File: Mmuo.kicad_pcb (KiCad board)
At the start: 4 copper layers, 95 parts, among them IC1 A121-001-T&R, IC2 BQ24253RGER, IC3 ADPL40502AUJZ-1.8-R7, J1 USB_C_Receptacle_USB2.0_16P, J2 B2B-PH-K-S, J3 SW_Debug, Q1 BSS84, Q2 BSS138, Q3 MMBT3904, SW1 PTS815, U1 USBLC6-2SC6, U2 RT9166A-33GXL, U3 EKMB1309113K, U4 STM32WB55CGU6, U5 MCP9808_MSOP, Y1 24MHz, Y2 32MHz, Y3 32K768

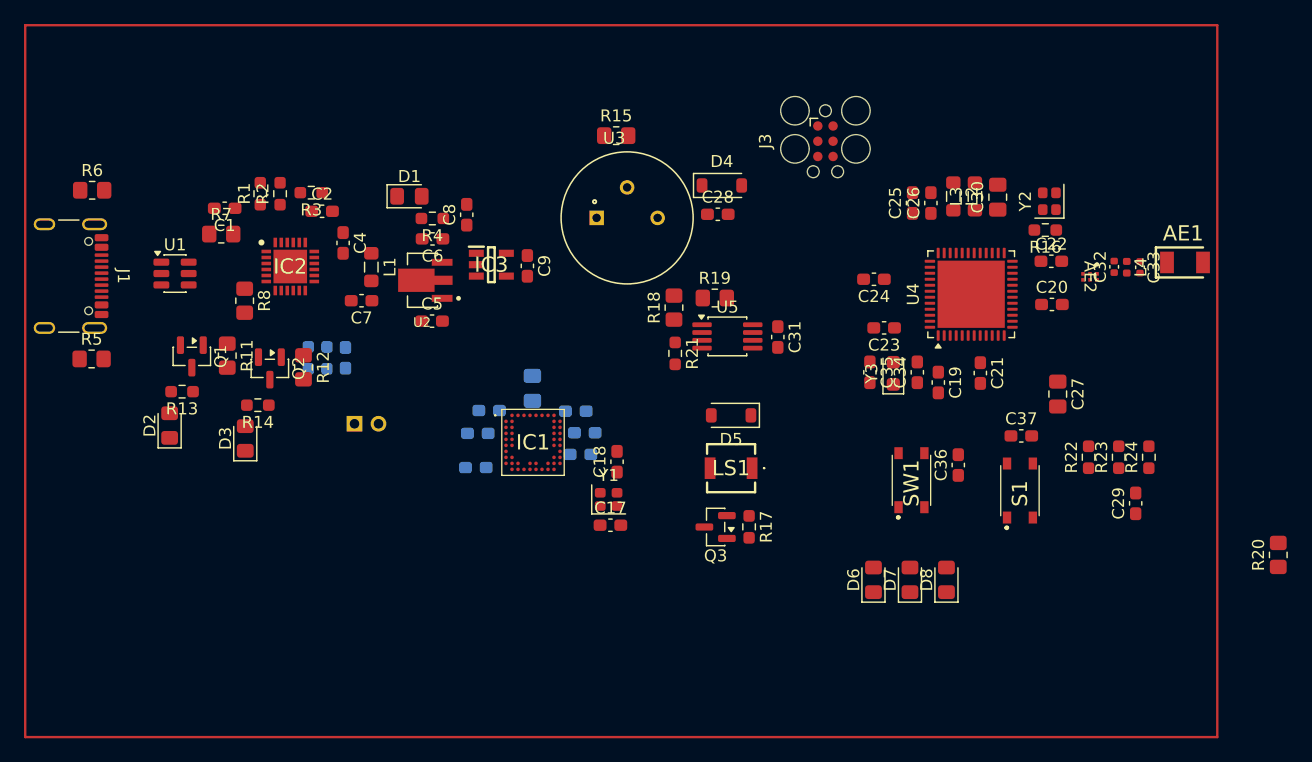
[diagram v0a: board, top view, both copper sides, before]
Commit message: Layout and initial routing
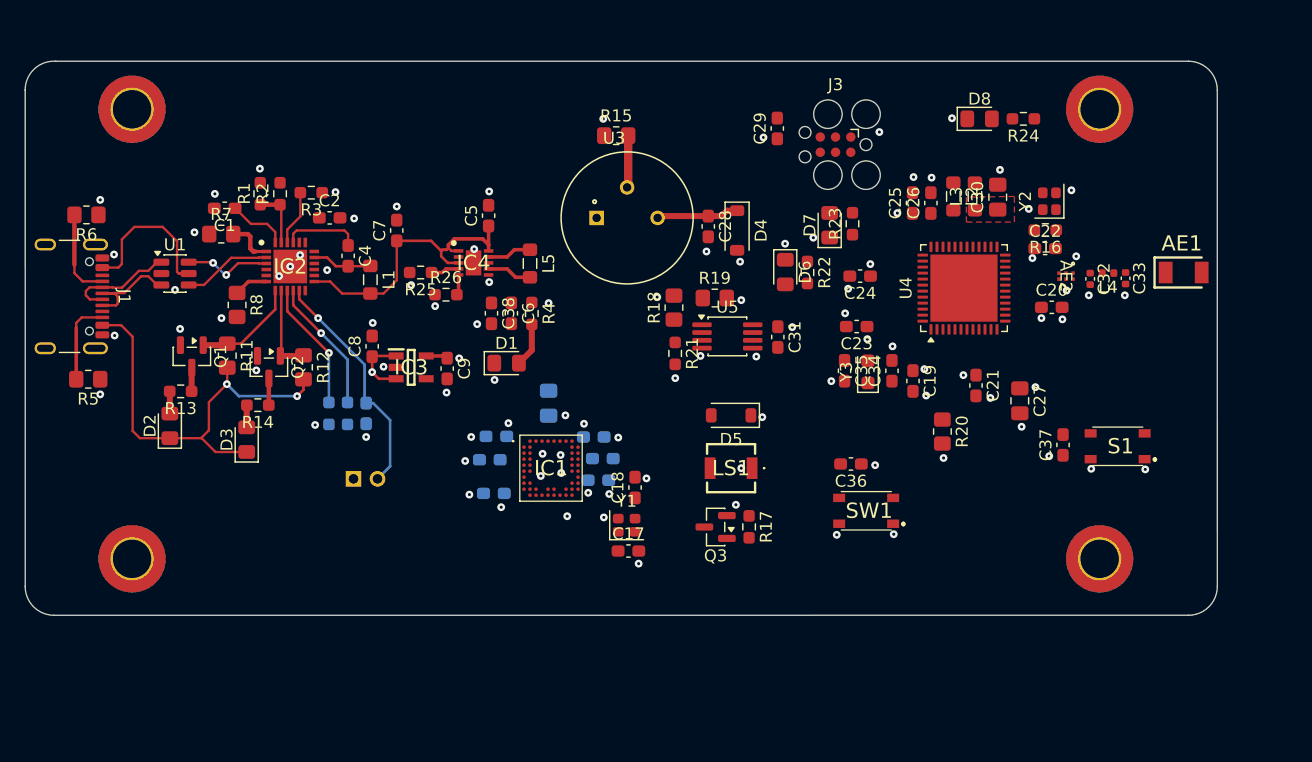
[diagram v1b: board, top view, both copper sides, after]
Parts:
- removed U2: RT9166A-33GXL, RT9166A_33GXL:VREG_AP7370-33Y-13
- added C38: 10u, Capacitor_SMD:C_0603_1608Metric_Pad1.08x0.95mm_HandSolder, F.Cu at (139.5, 102.8)
- added H1: MountingHole_Pad, MountingHole:MountingHole_3.2mm_M3_DIN965_Pad_TopBottom, F.Cu at (109.6, 85.8)
- added H2: MountingHole_Pad, MountingHole:MountingHole_3.2mm_M3_DIN965_Pad_TopBottom, F.Cu at (109.6, 123.2)
- added H3: MountingHole_Pad, MountingHole:MountingHole_3.2mm_M3_DIN965_Pad_TopBottom, F.Cu at (190.2, 123.2)
- added H4: MountingHole_Pad, MountingHole:MountingHole_3.2mm_M3_DIN965_Pad_TopBottom, F.Cu at (190.2, 85.8)
- added IC4: RAA2361052GNP#HC5, RAA2361052GNP:SON50P250X250X90-11N-D, F.Cu at (138.1, 98.6)
- added L5: 1u, Inductor_SMD:L_0805_2012Metric_Pad1.05x1.20mm_HandSolder, F.Cu at (142.8, 98.6)
- added R25: 0, Resistor_SMD:R_0603_1608Metric_Pad0.98x0.95mm_HandSolder, F.Cu at (133.6, 99.4)
- added R26: 332k, Resistor_SMD:R_0603_1608Metric_Pad0.98x0.95mm_HandSolder, F.Cu at (135.8, 101.2)
- C5, C6: value 1u -> 10u
- moved C29 43.2 mm to (163.3, 87.4)
- moved D8 38.5 mm to (180.2, 86.6), turned to 0 degrees
- moved D7 30.3 mm to (167.7, 95.5)
- moved R24 30.1 mm to (183.8, 86.6), turned to 180 degrees
- moved R20 29.8 mm to (177.1, 112.6), turned to -90 degrees
- moved R23 29.5 mm to (169.6, 95.3)
- moved R22 28.0 mm to (165.9, 99.4), turned to -90 degrees
- moved D6 26.7 mm to (164.0, 99.4), turned to -90 degrees
- moved D1 16.1 mm to (140.8, 106.9)
- moved C8 13.5 mm to (129.6, 105.5)
- moved R4 11.5 mm to (142.9, 102.8), turned to -90 degrees
- moved IC3 10.9 mm to (132.8, 107.3)
- moved C9 10.9 mm to (135.8, 107.4)
- moved C5 9.97 mm to (139.3, 94.7), turned to 90 degrees
- moved C6 9.03 mm to (141.2, 102.8), turned to -90 degrees
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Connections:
- net /USB_ESD_M renamed /USB_ESD_N
- net /USB_M renamed /USB_N
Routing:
- net +5V: track 0.00 -> 48.6 mm, vias 0 -> 2
- net Net-(IC2-SYS_1): track 0.00 -> 24.9 mm
- net Net-(IC2-BAT_1): track 0.00 -> 19.6 mm, vias 0 -> 1
- net +3V3: track 0.00 -> 12.4 mm, vias 0 -> 20
- net Net-(IC2-ISET): track 0.00 -> 11.2 mm, vias 0 -> 1
- net Net-(IC2-TS): track 0.00 -> 10.8 mm, vias 0 -> 1
- net /USB_N: track 0.00 -> 9.18 mm
- net /USB_P: track 0.00 -> 9.12 mm
- net /~{CHG}: track 0.00 -> 8.80 mm
- net /CC1: track 0.00 -> 7.46 mm
- net /~{PG}: track 0.00 -> 7.43 mm
- net /USB_ESD_P: track 0.00 -> 7.41 mm
- net /USB_ESD_N: track 0.00 -> 7.32 mm, vias 0 -> 2
- net /CC2: track 0.00 -> 7.06 mm
- net /BT: track 0.00 -> 6.49 mm
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- added copper zone on In2.Cu, net +1V8
- added copper zone on In2.Cu, net +3V3
- added copper zone on F.Cu, net /SMPSFB
- added copper zone on In1.Cu, net GND
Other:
- board outline added: 99.3 x 46.2 mm
